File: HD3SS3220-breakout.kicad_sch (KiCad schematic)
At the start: 32 parts, among them J1 USB_C_Receptacle, J2 U-A-39SS-Y-1, J3 A2541WV-2x4P, SW1 DSHP06TSGER_C3293146, U1 HD3SS3220RNHR, U2 TPD2EUSB30, U3 TPD4EUSB30, U4 HT7533-1_C14289

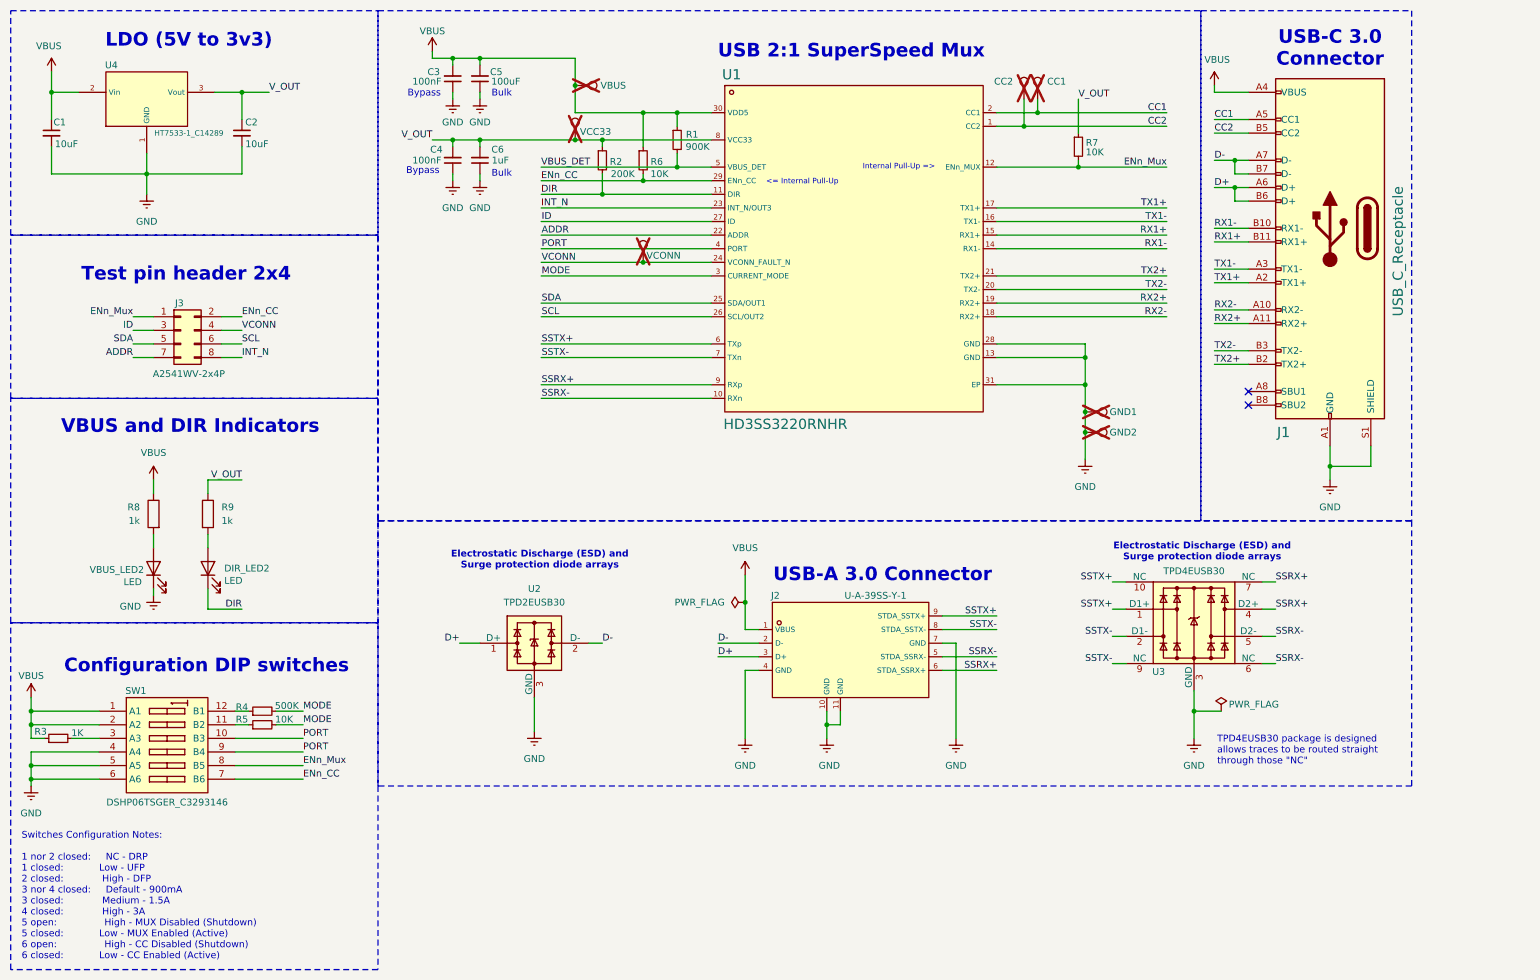
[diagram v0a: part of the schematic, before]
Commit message: Corrected ESD Diodes logic
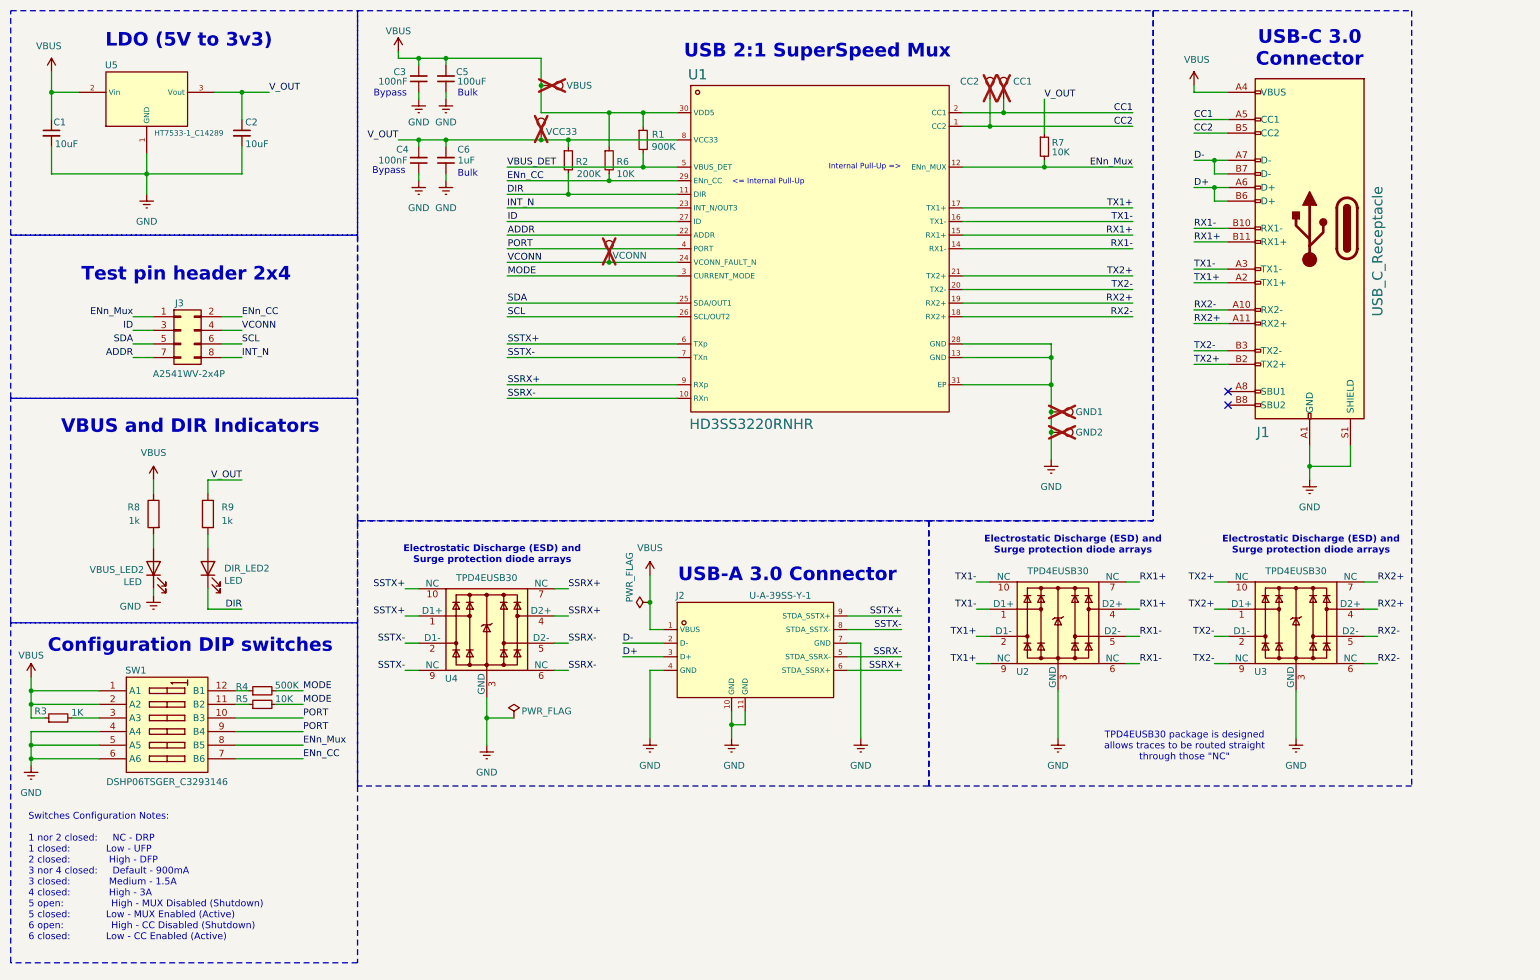
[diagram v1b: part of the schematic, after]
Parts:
- removed U2: TPD2EUSB30, Package_TO_SOT_SMD:Texas_DRT-3, symbol Power_Protection:TPD2EUSB30
- added U2, U3: TPD4EUSB30, Package_SON:USON-10_2.5x1.0mm_P0.5mm, symbol Power_Protection:TPD4EUSB30
- renumbered U3 to U4, U4 to U5
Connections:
- net GND: now also U2.3 (GND), U2.8 (GND), U3.3 (GND), U3.8 (GND)
- net RX1+: now also U2.4 (D2+), U2.7 (NC)
- net RX1-: now also U2.5 (D2-), U2.6 (NC)
- net RX2+: now also U3.4 (D2+), U3.7 (NC)
- net RX2-: now also U3.5 (D2-), U3.6 (NC)
- net TX1+: now also U2.2 (D1-), U2.9 (NC)
- net TX1-: now also U2.1 (D1+), U2.10 (NC)
- net TX2+: now also U3.1 (D1+), U3.10 (NC)
- net TX2-: now also U3.2 (D1-), U3.9 (NC)
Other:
- moved on the sheet: C3, C4, C5, C6, J1, J2, R1, R2, R3, R4, R5, R6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
